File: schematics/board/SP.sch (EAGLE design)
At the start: 20 parts

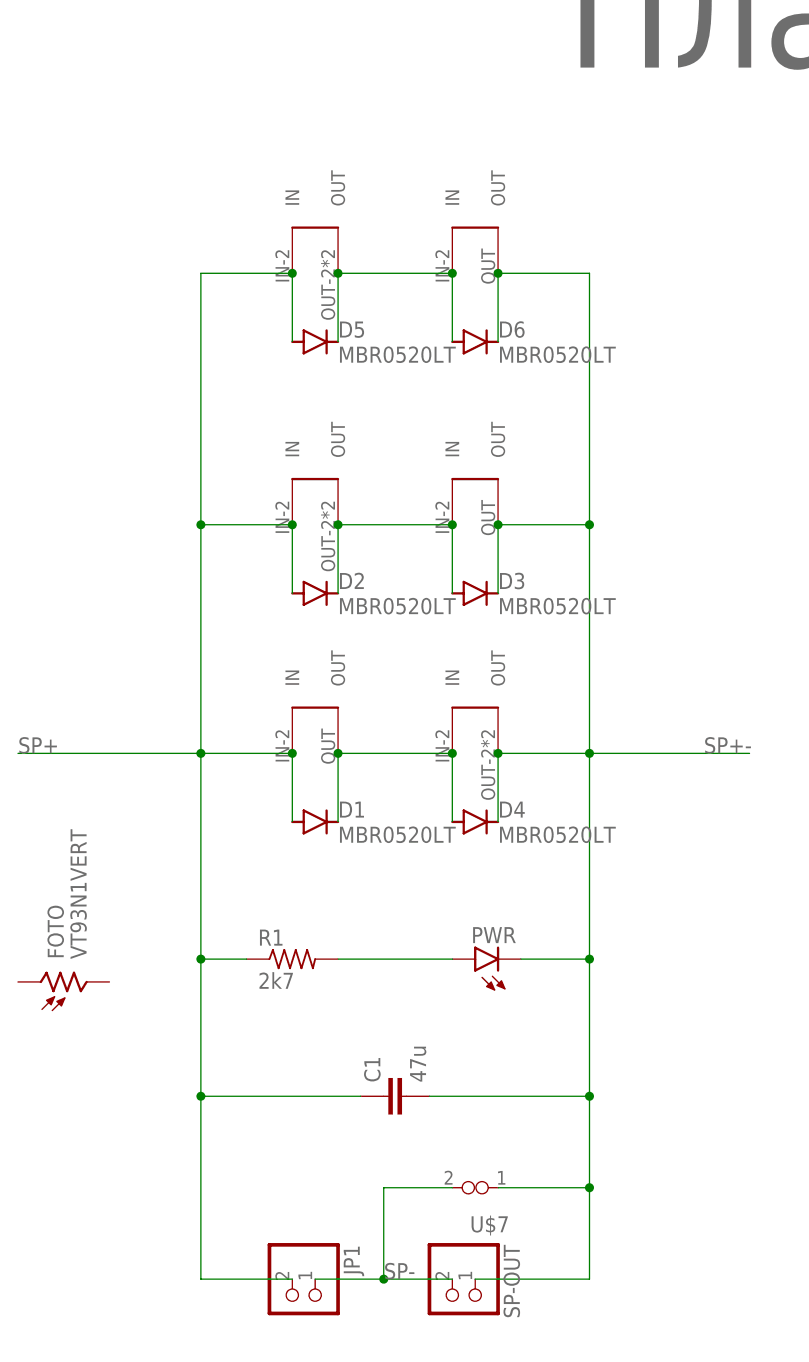
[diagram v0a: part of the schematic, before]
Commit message: Платы готовы
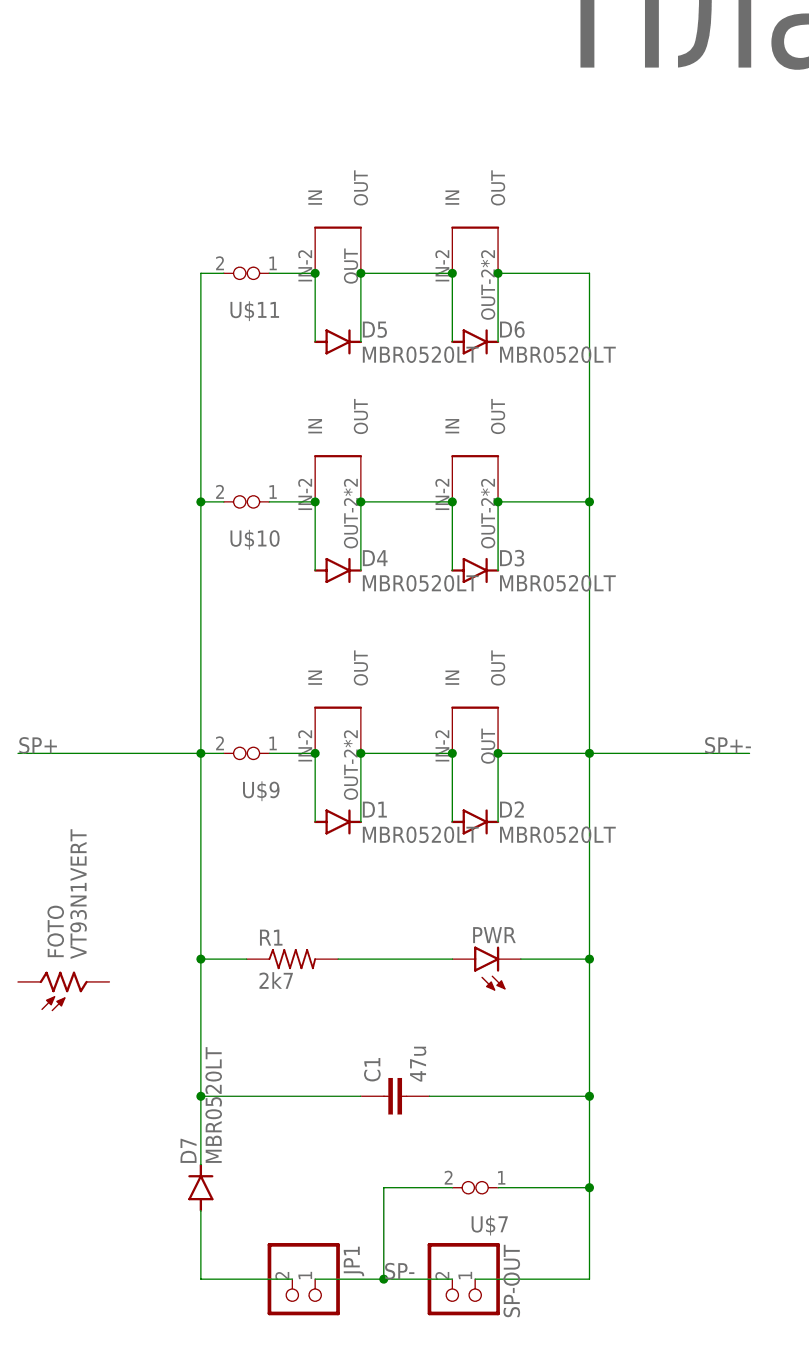
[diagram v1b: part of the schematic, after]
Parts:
- added D7: MBR0520LT, diode:MBR0520LT
- added U$10, U$11, U$9: (no value), KNPN-2023:VIAS-CONNECT
- U$1, U$3, U$8: value SOLAR-2_1 -> SOLAR-2_INVERT0-2; device KNPN-2023:SOLAR-2_1 -> KNPN-2023:SOLAR-2_INVERT0-2
- U$2, U$6: value SOLAR-2_0 -> SOLAR-2_INVERT1-2; device KNPN-2023:SOLAR-2_0 -> KNPN-2023:SOLAR-2_INVERT1-2
- U$4: value SOLAR-2_0 -> SOLAR-2_INVERT0-2; device KNPN-2023:SOLAR-2_0 -> KNPN-2023:SOLAR-2_INVERT0-2
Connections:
- new net N$1: D7.A, JP1.2
- new net N$5: D1.C, D2.A, U$1.OUT, U$2.IN
- new net N$6: D3.A, D4.C, U$3.IN, U$4.OUT
- new net N$7: D1.A, U$1.IN, U$9.1
- net N$2: now also D5.A, U$11.1, U$6.IN; no longer D2.C, D3.A, U$2.OUT, U$3.IN
- net N$3: now also U$10.1; no longer D1.C, U$1.OUT
- net SP+: now also D7.C, U$10.2, U$11.2, U$9.2; no longer D1.A, D2.A, D5.A, JP1.2, U$1.IN, U$2.IN, U$6.IN
- net SP+-: now also D2.C, U$2.OUT; no longer D4.C, U$4.OUT
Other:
- moved on the sheet: D1, D2, D3, D4, D5
